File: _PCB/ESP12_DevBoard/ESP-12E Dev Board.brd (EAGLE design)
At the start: 70 x 70 mm, 48 parts, among them J1 ZX62-B-5PA(33), J10 DUST_SENSOR, J2 I2C, J3 LCD, J4 I2C, J5 LCD_BACKLIGHT, J6 TEMP/HUM SENSOR, J7 RADON_SENSOR, J8 BUTTON1, J9 ADC, Q1 UMH3N, U1 5V_REG, U2 3.3V_REG, U3 CH340C, U4 TXB0104

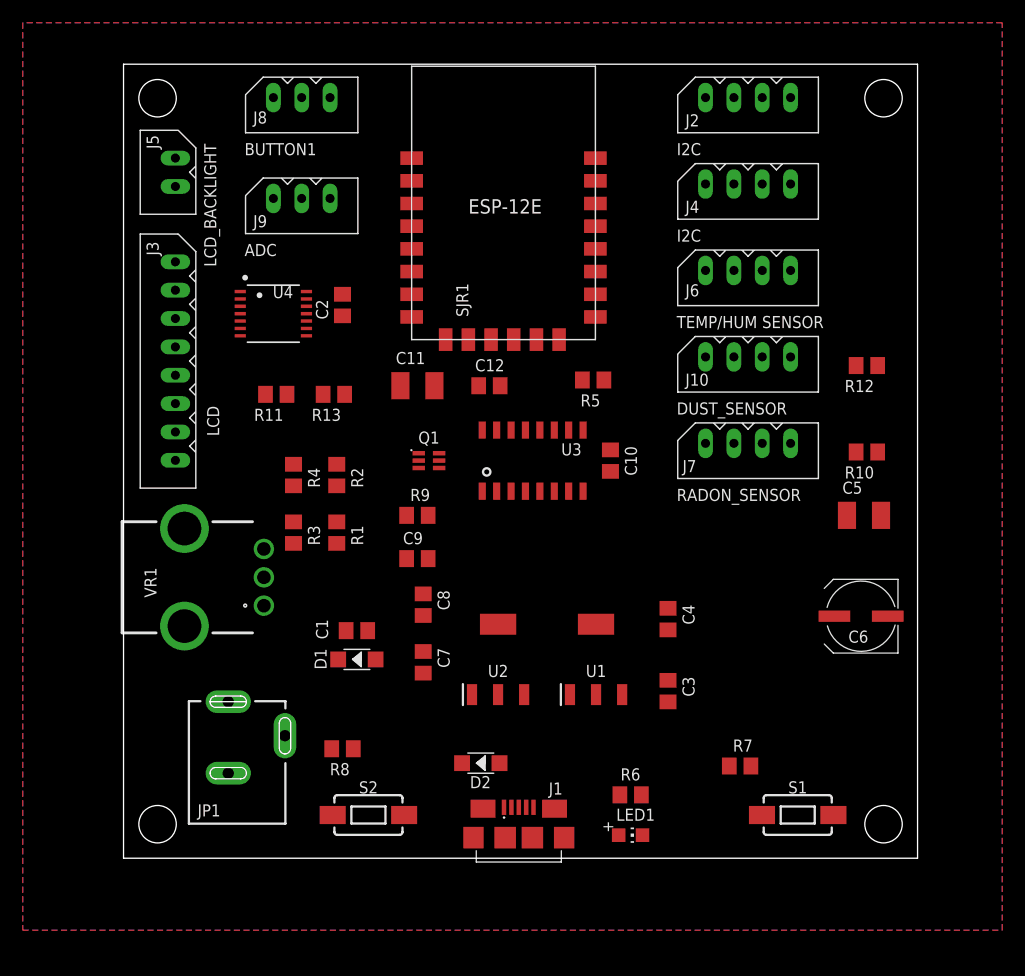
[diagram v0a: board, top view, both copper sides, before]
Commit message: PCB layout V1
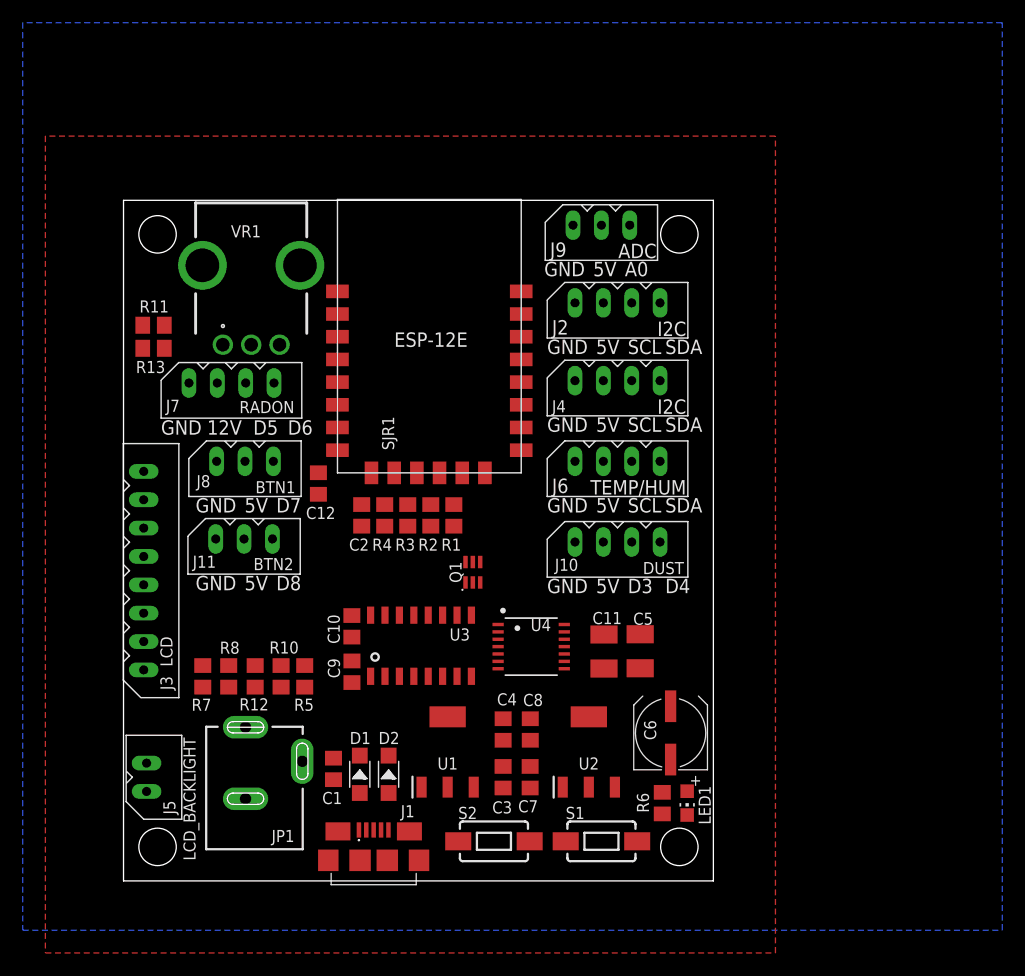
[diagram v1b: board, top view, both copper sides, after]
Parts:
- removed R9: 470Ω, rcl:R0805
- added J11: BTN2, con-molex-spox:5267-3
- J10: value DUST_SENSOR -> DUST
- J6: value TEMP/HUM SENSOR -> TEMP/HUM
- J7: value RADON_SENSOR -> RADON
- J8: value BUTTON1 -> BTN1
- U2: value 3.3V_REG -> 3V3_REG
- moved R12 60.5 mm to (11.6, 16.0), turned to 270 degrees
- moved J5 55.9 mm to (2.03, 5.89), turned to 90 degrees
- moved R10 55.3 mm to (13.9, 16.0), turned to 270 degrees
- moved R7 48.0 mm to (6.99, 16.0), turned to 270 degrees
- moved J7 45.9 mm to (5.76, 41.9)
- moved U4 37.1 mm to (35.9, 18.7)
- moved R5 36.5 mm to (16.0, 16.0), turned to 90 degrees
- moved J3 36.1 mm to (1.78, 16.6), turned to 90 degrees
- moved VR1 34.9 mm to (11.3, 57.8), turned to 0 degrees
- moved J8 32.5 mm to (8.21, 35.0)
- moved C11 28.6 mm to (42.4, 18.2), turned to 270 degrees
- moved C10 27.1 mm to (20.1, 20.4), turned to 90 degrees
- moved J9 26.5 mm to (39.6, 55.8)
- moved C5 23.1 mm to (45.5, 18.2), turned to 270 degrees
- moved J2 21.4 mm to (39.8, 49.0)
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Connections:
- removed net 12V_INPUT: D1.+, JP1.PWR
- removed net LED+_5V: J5.P$2, U4.11
- removed net LED-_5V: U4.10
- new net LED+: J3.P$7, J5.P$2
- new net RXD_5V: U3.2, U4.10
- new net TXD_5V: U3.3, U4.11
- net 12V: no longer C1.2
- net 3.3V: no longer J8.P$2
- net 5V: now also J11.P$2, J8.P$2
- net GND: now also J11.P$1, J3.P$8
- net GPIO0: now also R12.1; no longer U4.4
- net GPIO12: now also J7.P$4; no longer R10.1
- net GPIO13: now also J8.P$3; no longer J7.P$4
- net GPIO14: now also R10.1; no longer R12.1
- net GPIO15: now also J11.P$3; no longer J8.P$3
- net GPIO16: no longer J10.P$4
- net GPIO2: now also J10.P$4; no longer U4.5
- net N$3: now also C1.2, D1.+, JP1.PWR; no longer R9.2, U3.2
- net RXD: now also U4.5; no longer R9.1
- net TXD: now also U4.4; no longer U3.3
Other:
- board size 70 x 70 mm -> 52 x 60 mm
- board text added: "12V"
- board text added: "5V"
- board text added: "A0"
- board text added: "D3"
- board text added: "D4"
- board text added: "D5"
- board text added: "D6"
- board text added: "D7"
- board text added: "D8"
- board text added: "GND"
- board text added: "SCL"
- board text added: "SDA"
